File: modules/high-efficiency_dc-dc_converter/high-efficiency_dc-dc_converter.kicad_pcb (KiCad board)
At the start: 2 copper layers, 27.9 x 20.3 mm, 13 parts

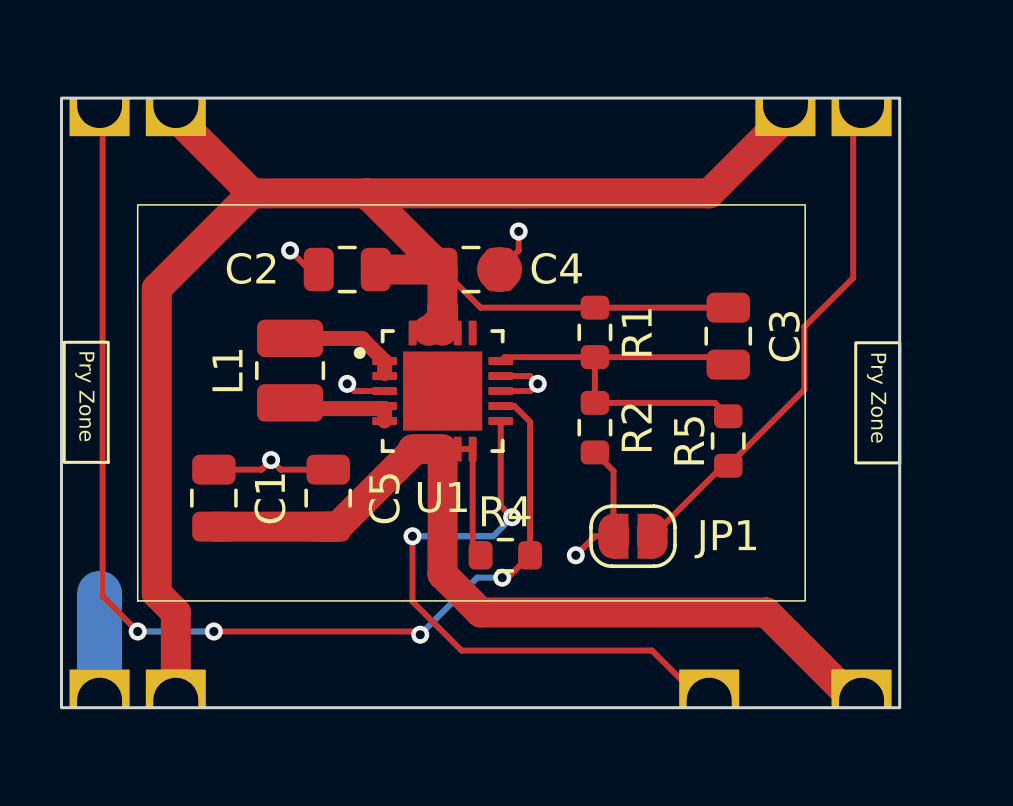
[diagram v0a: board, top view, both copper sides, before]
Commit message: add silkscreen hints etc to 2A DC:DC Module
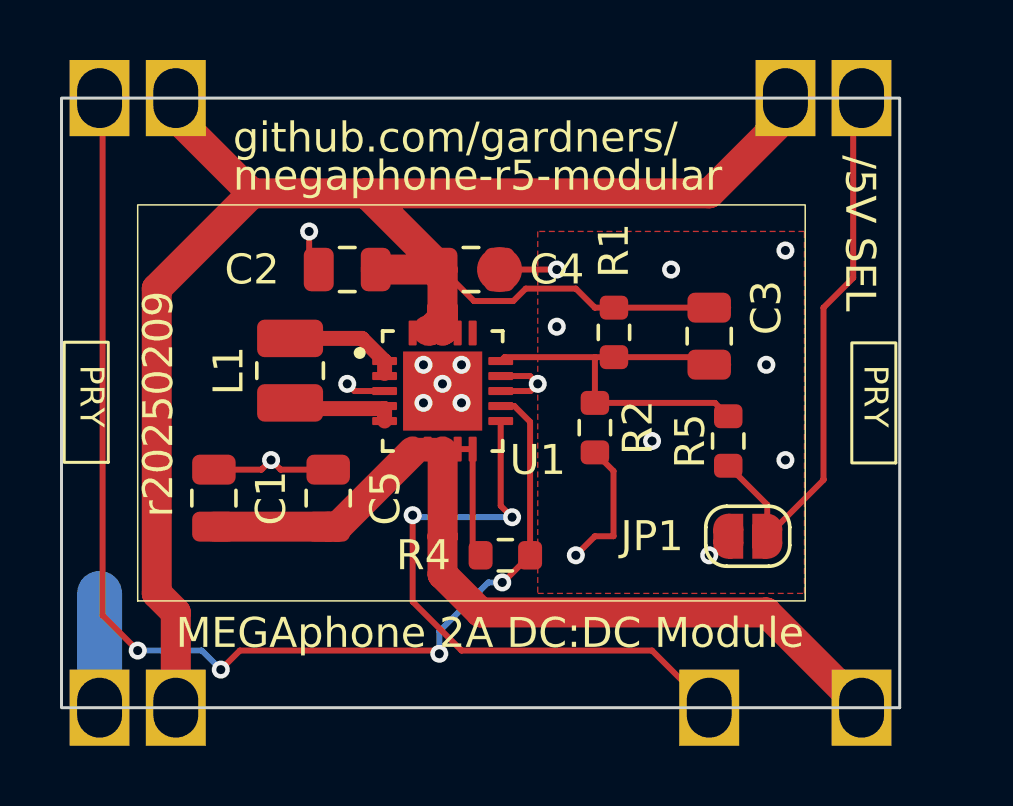
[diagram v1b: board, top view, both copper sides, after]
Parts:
- moved JP1 3.83 mm to (72.4, 45.1)
- moved C3 0.63 mm to (71.1, 38.4)
- moved R1 0.63 mm to (67.9, 38.3)
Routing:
- net MODE: track 38.4 -> 40.2 mm
- net /5V_SEL: track 17.6 -> 19.0 mm
- net GND: track 19.2 -> 19.8 mm, vias 6 -> 18
- added copper zone on F.Cu, net GND
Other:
- board text added: "/5V SEL"
- board text added: "MEGAphone 2A DC:DC Module"
- board text added: "U1 ISL91127IRAZ"
- board text added: "github.com/gardners/"
- board text added: "megaphone-r5-modular"
- board text added: "r20250209"
